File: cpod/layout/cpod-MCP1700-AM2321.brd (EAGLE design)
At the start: 13 parts

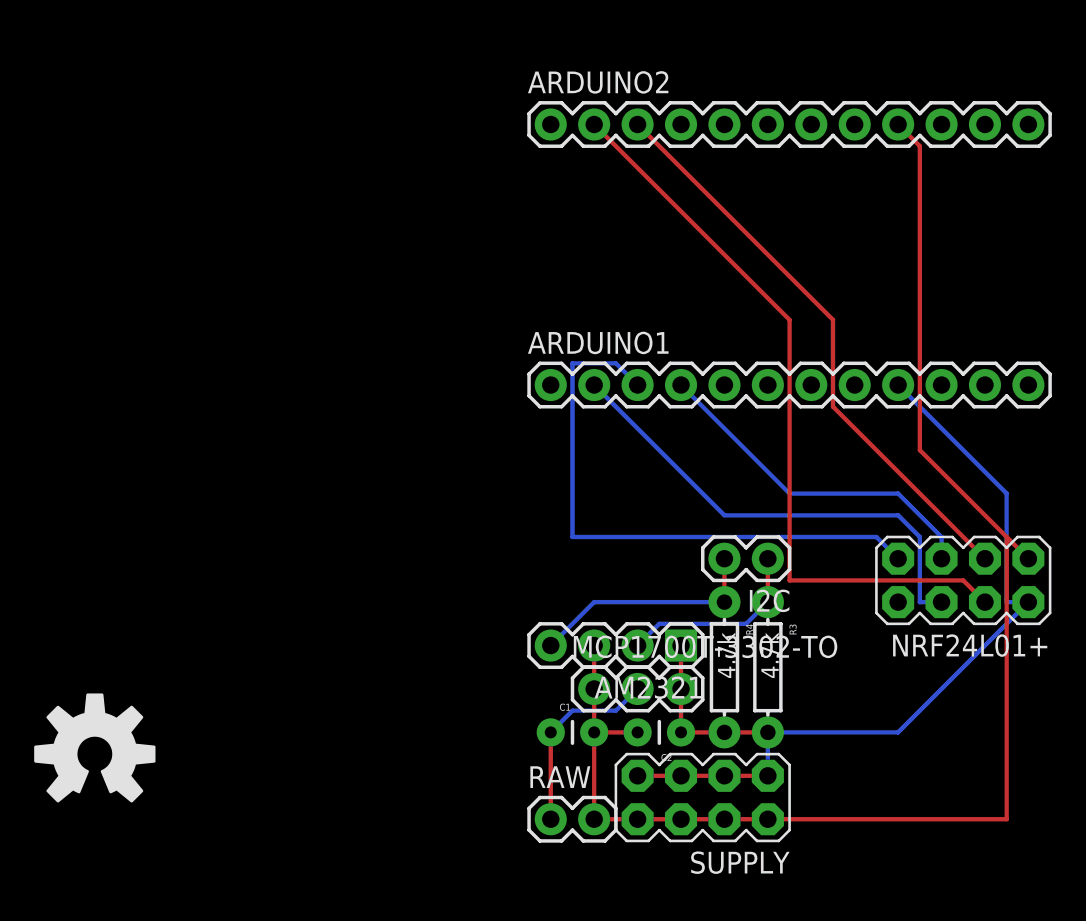
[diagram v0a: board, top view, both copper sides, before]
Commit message: 布线完成
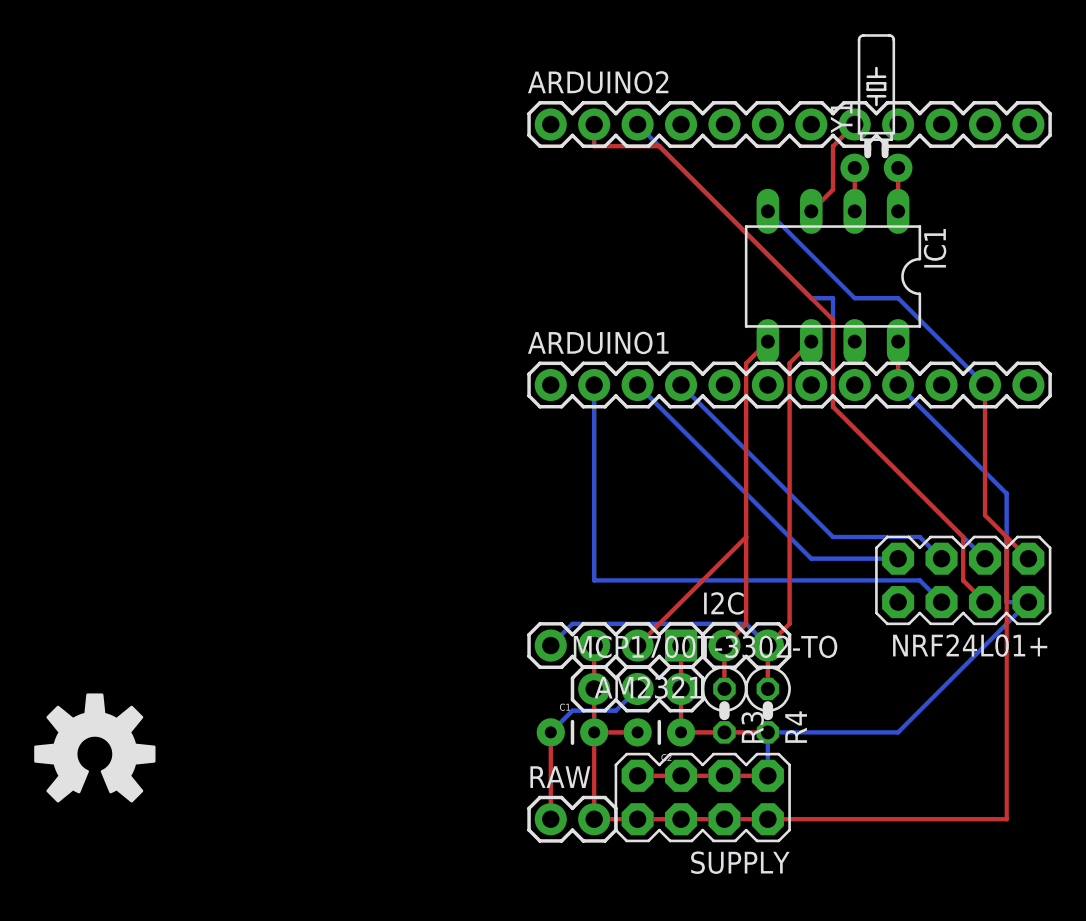
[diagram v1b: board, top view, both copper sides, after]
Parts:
- added IC1: PCF8563DIP, CEDT:DIL08
- added Y1: 32.768kHz, SparkFun-FreqCtrl:TC26H
- R3, R4: device SparkFun-Resistors:AXIAL-0.3 -> rcl:0207/2V
- moved I2C 5.68 mm to (41.9, -31.8), turned to 0 degrees
- moved R3 3.59 mm to (41.9, -35.6)
- moved R4 3.59 mm to (44.5, -35.6)
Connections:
- removed net D2: ARDUINO2.8
- new net INT0: ARDUINO2.8, IC1.3
- new net N$4: IC1.1, Y1.2
- new net N$6: IC1.2, Y1.1
- net GND: now also ARDUINO1.11, IC1.4; no longer ARDUINO2.9
- net SCL: now also IC1.6, R4.1; no longer R4.P$1
- net SDA: now also IC1.5, R3.1; no longer R3.P$1
- net VCC: now also IC1.8, R3.2, R4.2; no longer R3.P$2, R4.P$2
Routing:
- net SCL: track 13.8 -> 35.1 mm
- net SDA: track 11.2 -> 30.4 mm
- net MISO: track 34.1 -> 19.4 mm
- net INT0: track 0.00 -> 6.13 mm
- net MOSI: track 27.8 -> 32.3 mm
- net CSN: track 43.4 -> 39.6 mm
- net N$6: track 0.00 -> 2.54 mm
- net N$4: track 0.00 -> 2.54 mm
- net VCC: track 55.3 -> 57.9 mm
- net CE: track 33.8 -> 34.6 mm
- net SCK: track 20.2 -> 19.4 mm
